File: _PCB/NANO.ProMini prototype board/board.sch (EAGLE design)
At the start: 32 parts, among them T1_5MM 5mm, T2_5MM 5mm, T3_5MM 5mm

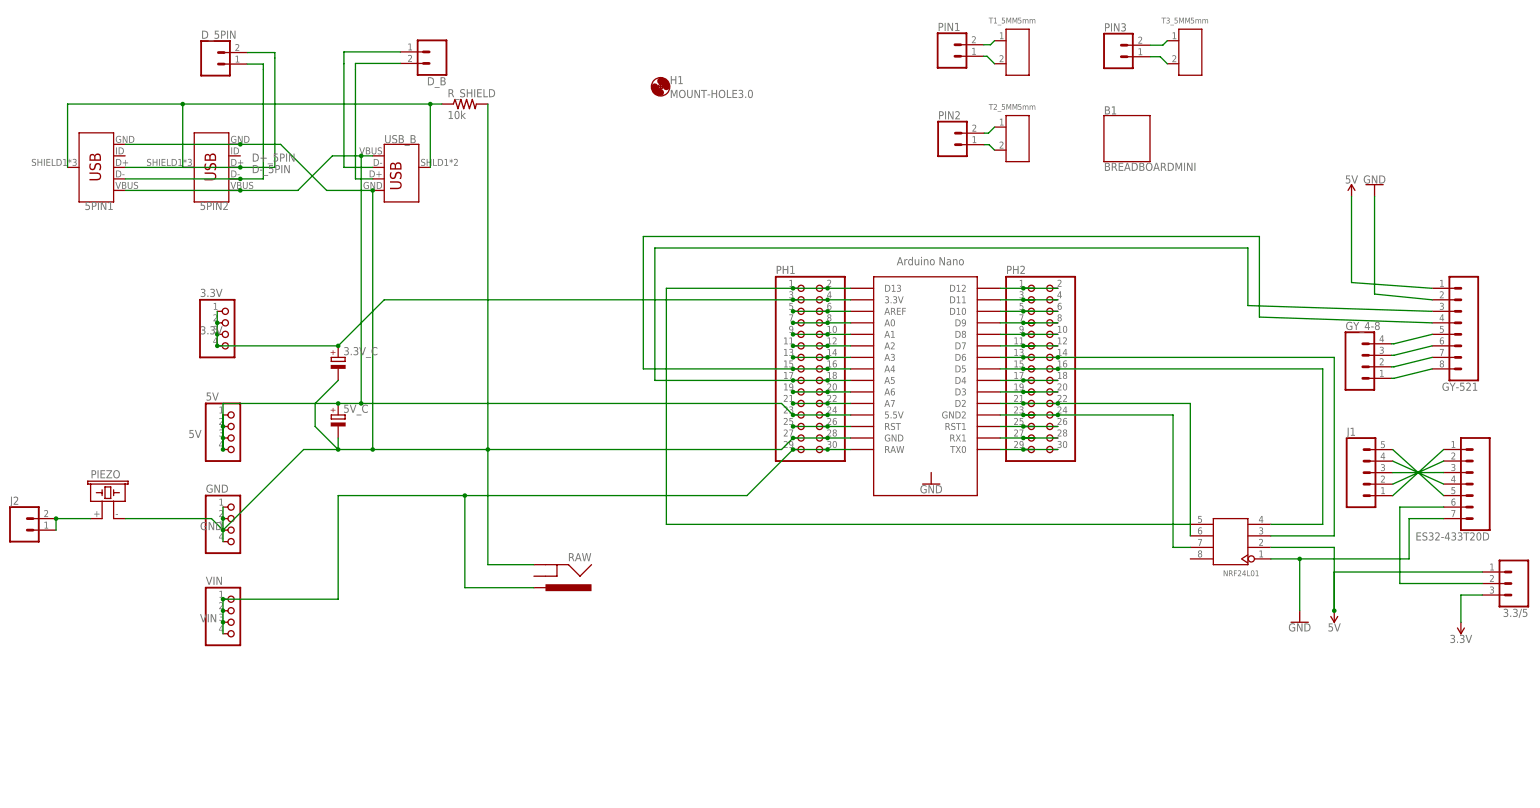
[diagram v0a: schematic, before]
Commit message: fixed issues - working version
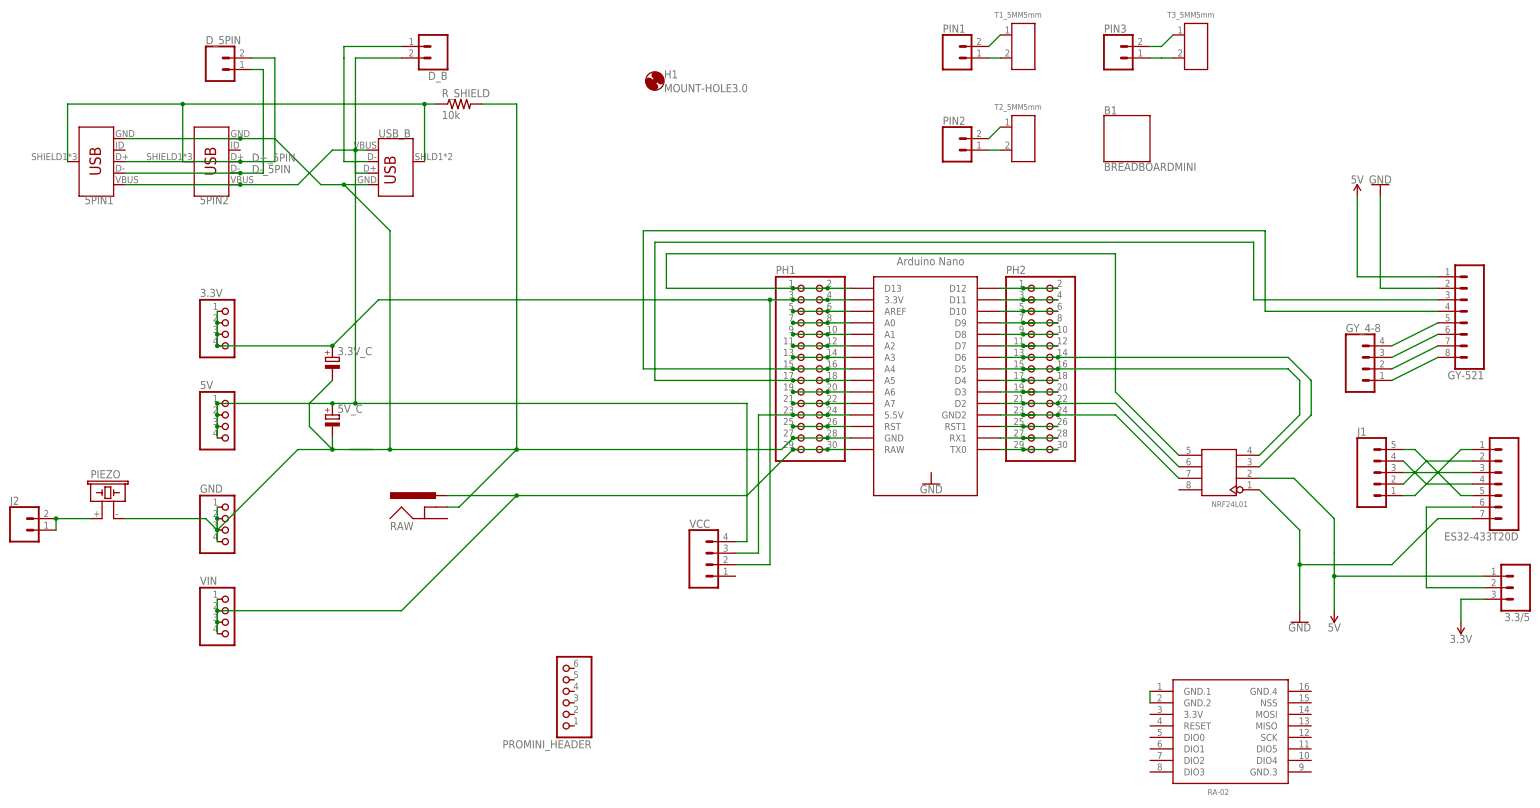
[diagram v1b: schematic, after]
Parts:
- added PROMINI_HEADER: (no value), pinhead_v2:PINHD-1X6/OCT
- added RA-02: LORA-RA-02-433MHZ, LikeCircuit:LORA-RA-02-433MHZ
- added VCC: (no value), SparkFun-Connectors:CONN_04LOCK_LONGPADS
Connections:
- new net N$1: RA-02.GND.1, RA-02.GND.2
- new net N$37: NANO.5.5V, PH1.23, PH1.24, VCC.3
- net 3.3V: now also VCC.2
- net 5V: now also VCC.4; no longer NANO.5.5V, PH1.23, PH1.24
- net GND: now also RAW.GNDBREAK; no longer RAW.GND
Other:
- moved on the sheet: 3.3/5, 3.3V_C, 5PIN1, 5PIN2, 5V, 5V_C, D_5PIN, D_B, ES32-433T20D, GND, GY-521, H1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
